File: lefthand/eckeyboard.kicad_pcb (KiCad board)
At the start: 2 copper layers, 135.8 x 94.3 mm, 60 parts, among them J4 Conn_01x06_Male, J5 Conn_01x06_Male, U1 74HC4051, U2 NJM2742, U4 74LS138

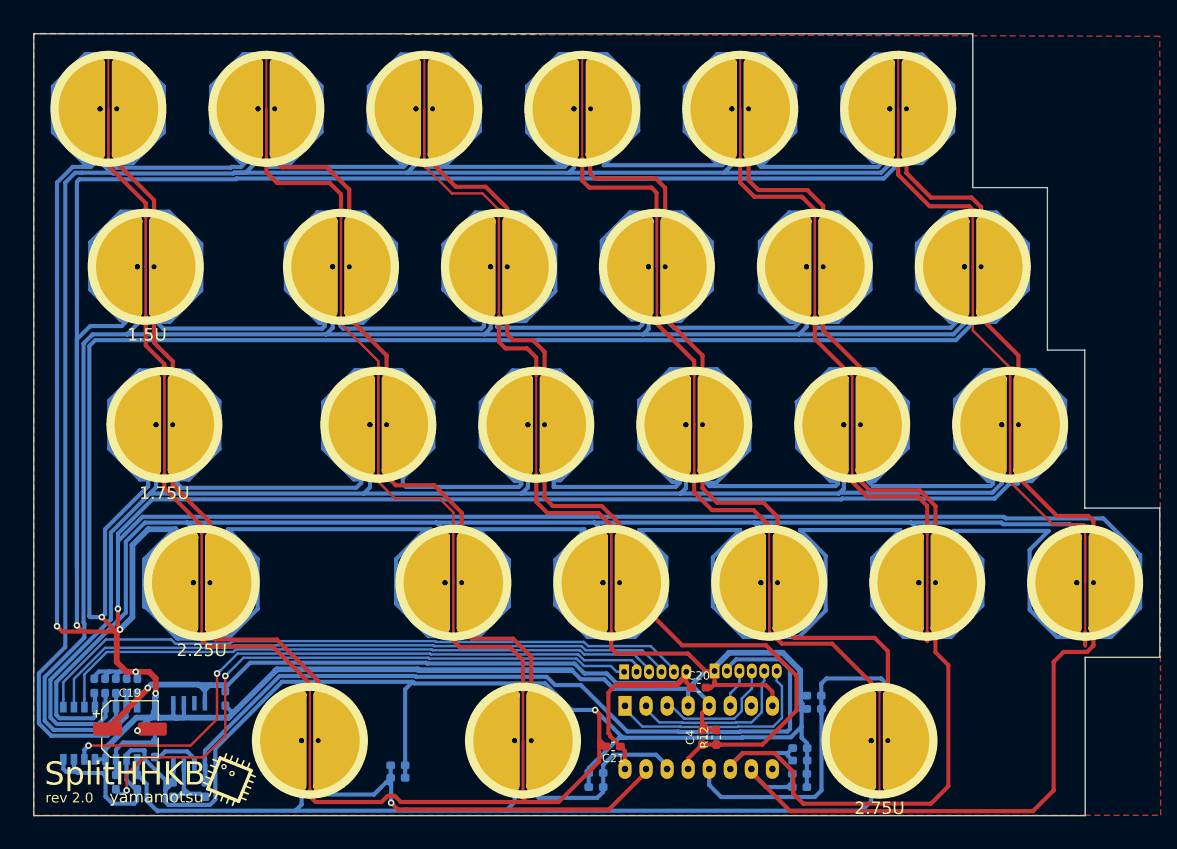
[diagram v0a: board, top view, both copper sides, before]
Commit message: [add] controller, righthand
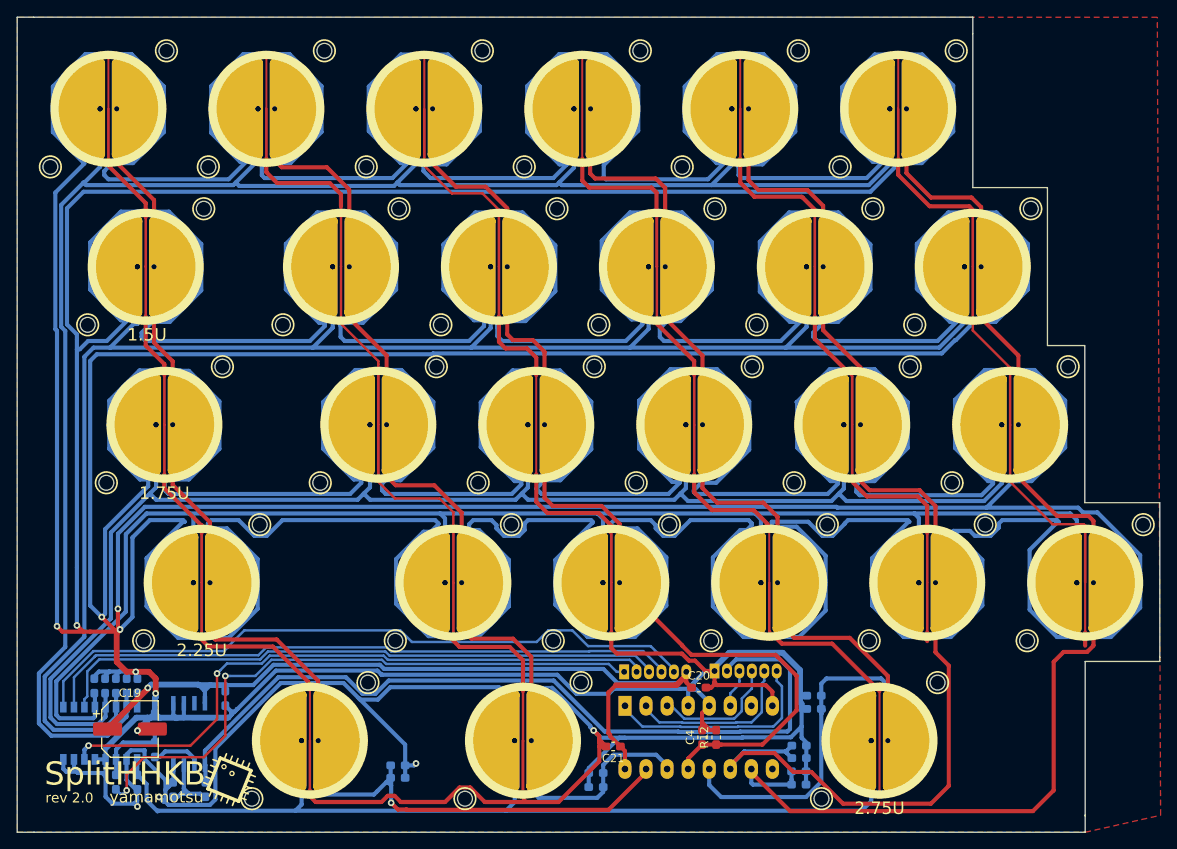
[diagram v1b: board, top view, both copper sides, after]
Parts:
- TP1, TP10, TP11, TP12, TP13, TP14, TP15, TP16, TP17, TP18, TP19, TP2, TP20, TP21, TP22, TP23, TP24, TP25, TP26, TP27, TP3, TP4, TP5, TP6, TP7, TP8, TP9: value ToprePad -> ToprePad_MntHole; footprint toprepad:ToprePad -> toprepad:ToprePad_MntHole
- moved C7 0.32 mm to (133.3, 129.9)
- moved R15 0.32 mm to (133.3, 131.5)
- moved C6 0.32 mm to (133.3, 126.8)
- moved R14 0.32 mm to (133.3, 128.3)
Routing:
- net GND: track 2927.1 -> 2891.3 mm, vias 9 -> 12
- net /ROW1: track 216.9 -> 227.5 mm
- net /ROW0: track 231.1 -> 238.4 mm
- net /ROW3: track 192.7 -> 199.8 mm
- net /ROW2: track 195.6 -> 198.9 mm
- net /COL3: track 149.5 -> 147.1 mm
- net /MUX_A: track 80.8 -> 82.7 mm
- net /READ: track 97.1 -> 98.3 mm
- net /COL4: track 141.3 -> 140.1 mm
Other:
- board size 135.8 x 94.3 mm -> 137.8 x 98.3 mm

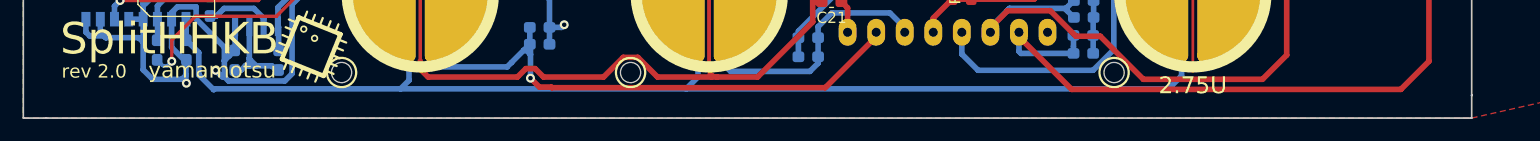
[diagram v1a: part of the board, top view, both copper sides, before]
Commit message: [add] step files
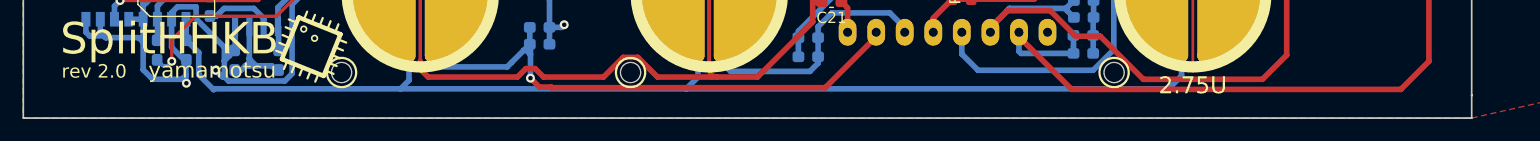
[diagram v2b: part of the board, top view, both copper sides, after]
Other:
- outline, holes or cut-outs redrawn
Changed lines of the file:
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@@
   (general
     (thickness 1.6)
-    (drawings 47)
+    (drawings 46)
     (tracks 1324)
     (zones 0)
@@
     (arrow2b (pts (xy 31.75 38.95) (xy 32.336421 40.076504)))
   )
-  (gr_line (start 39 137.25) (end 41.05 137.25) (layer Edge.Cuts) (width 0.15))
   (gr_line (start 39 38.95) (end 39 137.25) (layer Edge.Cuts) (width 0.15))
   (gr_line (start 41 38.95) (end 39 38.95) (layer Edge.Cuts) (width 0.15))
@@
   (gr_line (start 176.8 116.65) (end 176.8 116.15) (layer Edge.Cuts) (width 0.15))
   (gr_line (start 167.8 116.65) (end 176.8 116.65) (layer Edge.Cuts) (width 0.15))
-  (gr_line (start 167.8 137.25) (end 41 137.25) (layer Edge.Cuts) (width 0.15))
+  (gr_line (start 167.8 137.25) (end 39 137.25) (layer Edge.Cuts) (width 0.15))
   (gr_line (start 167.8 135.2) (end 167.8 135.25) (layer Edge.Cuts) (width 0.15))
   (gr_line (start 167.8 137.25) (end 167.8 135.2) (layer Edge.Cuts) (width 0.15))
